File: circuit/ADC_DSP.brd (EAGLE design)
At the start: 100 x 80 mm, 49 parts, among them IC1 REG1117, IC2 AD8605, IC3 STM32F40XRXT6, IC4 CS4272, Q1 8MHz, Q2 24.576MHz

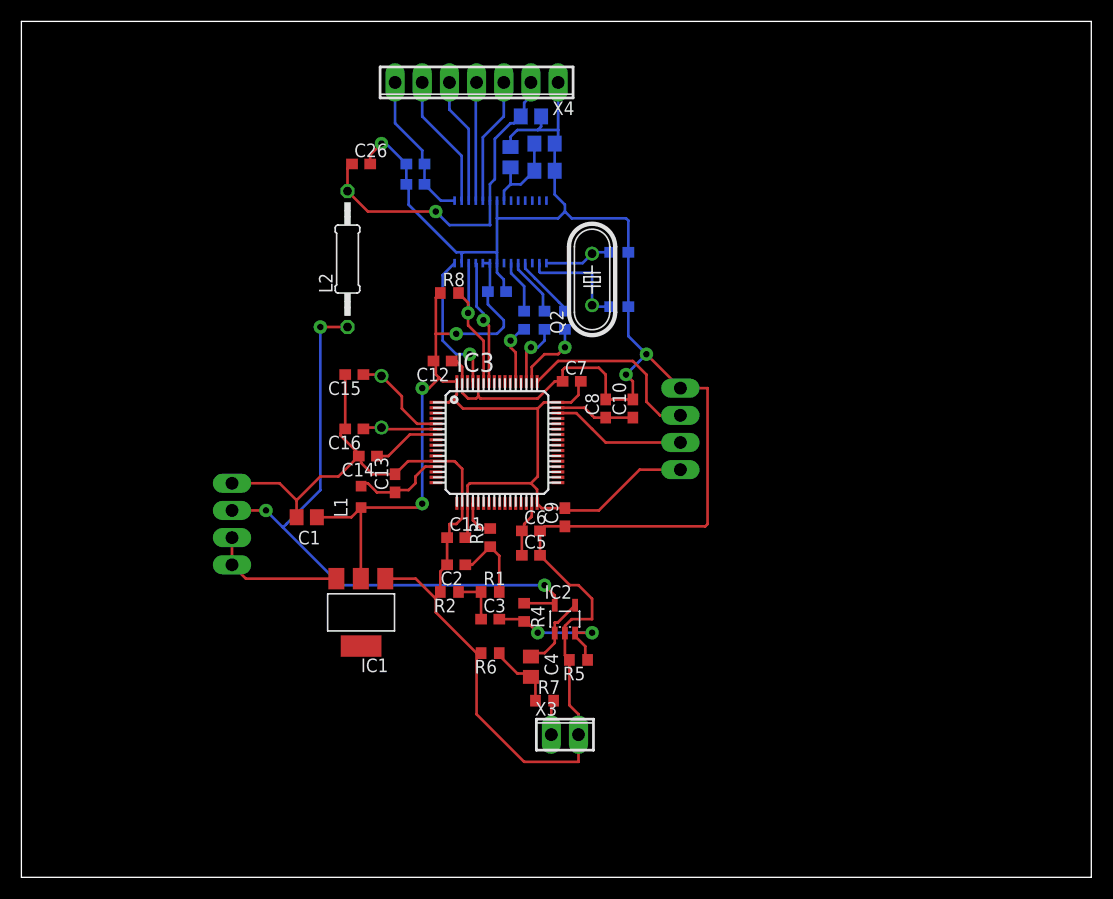
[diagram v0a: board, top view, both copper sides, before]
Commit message: - ??????? 51x57 ??
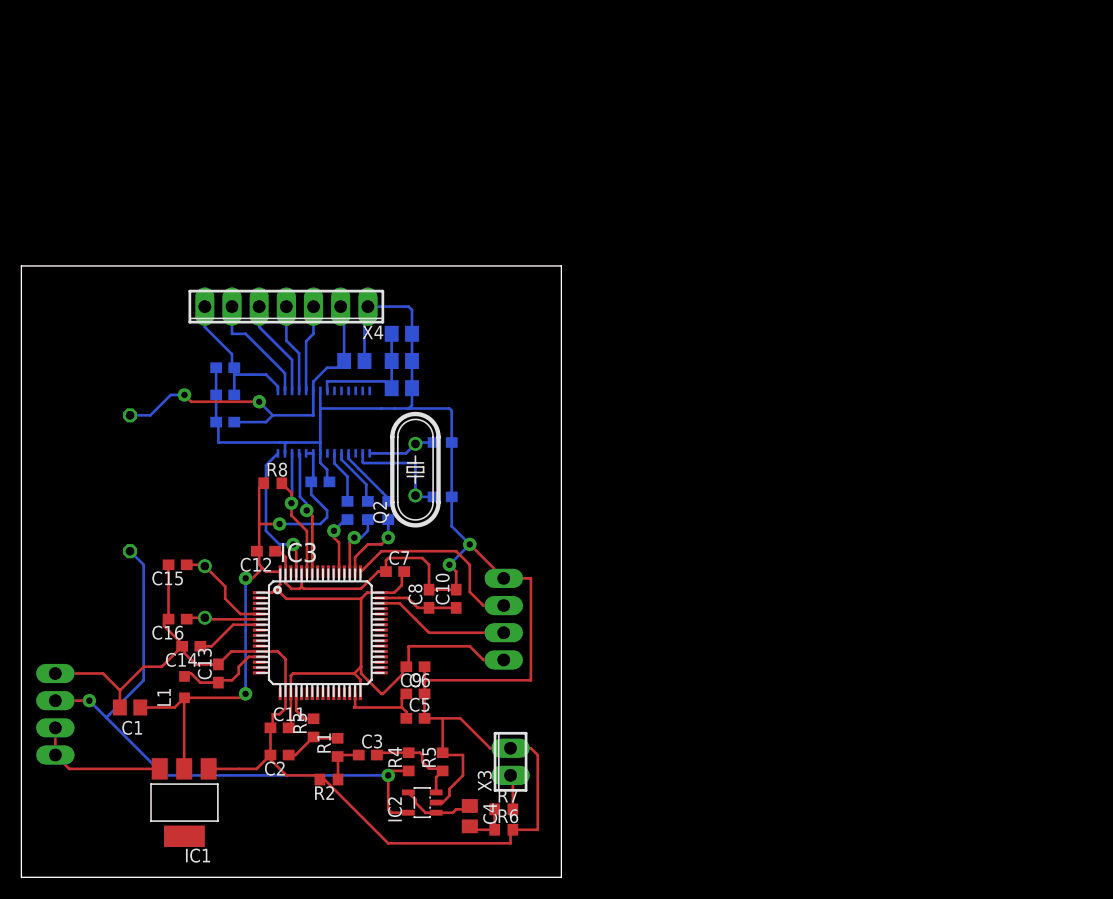
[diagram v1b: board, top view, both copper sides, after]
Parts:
- moved L2 29.2 mm to (10.2, 36.8), flipped to the bottom
- moved C25 28.2 mm to (31.1, 48.3)
- moved X4 27.5 mm to (24.8, 53.3)
- moved C26 27.3 mm to (19.1, 42.5), flipped to the bottom
- moved C20 26.5 mm to (19.1, 45.1)
- moved C22 26.1 mm to (19.1, 47.6)
- moved C23 24.3 mm to (35.6, 45.7)
- moved C24 24.3 mm to (35.6, 48.3)
- moved C18 24.3 mm to (39.4, 40.6)
- moved C19 24.3 mm to (39.4, 35.6)
- moved Q2 24.3 mm to (36.8, 38.1)
- moved R9 24.3 mm to (32.4, 34.3)
- moved C1 24.3 mm to (10.2, 15.9)
- moved C11 24.3 mm to (24.1, 14.0)
- moved C15 24.3 mm to (14.6, 29.2)
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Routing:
- net N$22: track 13.8 -> 9.70 mm, vias 2 -> 0
- net N$15: track 11.9 -> 8.16 mm
- net N$12: track 8.66 -> 12.3 mm
- net N$2: track 5.23 -> 8.40 mm
- net +3V3: track 107.3 -> 110.4 mm
- net N$16: track 11.1 -> 8.37 mm
- net N$17: track 11.8 -> 9.15 mm
- net N$23: track 7.61 -> 5.33 mm
- net N$14: track 32.5 -> 34.6 mm, vias 1 -> 2
- net N$20: track 6.40 -> 4.36 mm
- net N$18: track 12.6 -> 10.7 mm
- net GND: track 247.5 -> 245.6 mm, vias 3 -> 2
- net +5V: track 60.0 -> 58.8 mm, vias 3 -> 2
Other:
- board size 100 x 80 mm -> 50.5 x 57.1 mm
